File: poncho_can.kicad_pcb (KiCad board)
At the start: 2 copper layers, 85.7 x 60.3 mm, 33 parts, among them J10 GS2, J101 DB9_Male_MountingHoles, J102 DB9_Male_MountingHoles, J103 GS2, J104 GS2, J105 GS2, J106 GS2, J7 GS2, J8 GS2, J9 GS2, U101 TJA1051T, U102 TJA1051T

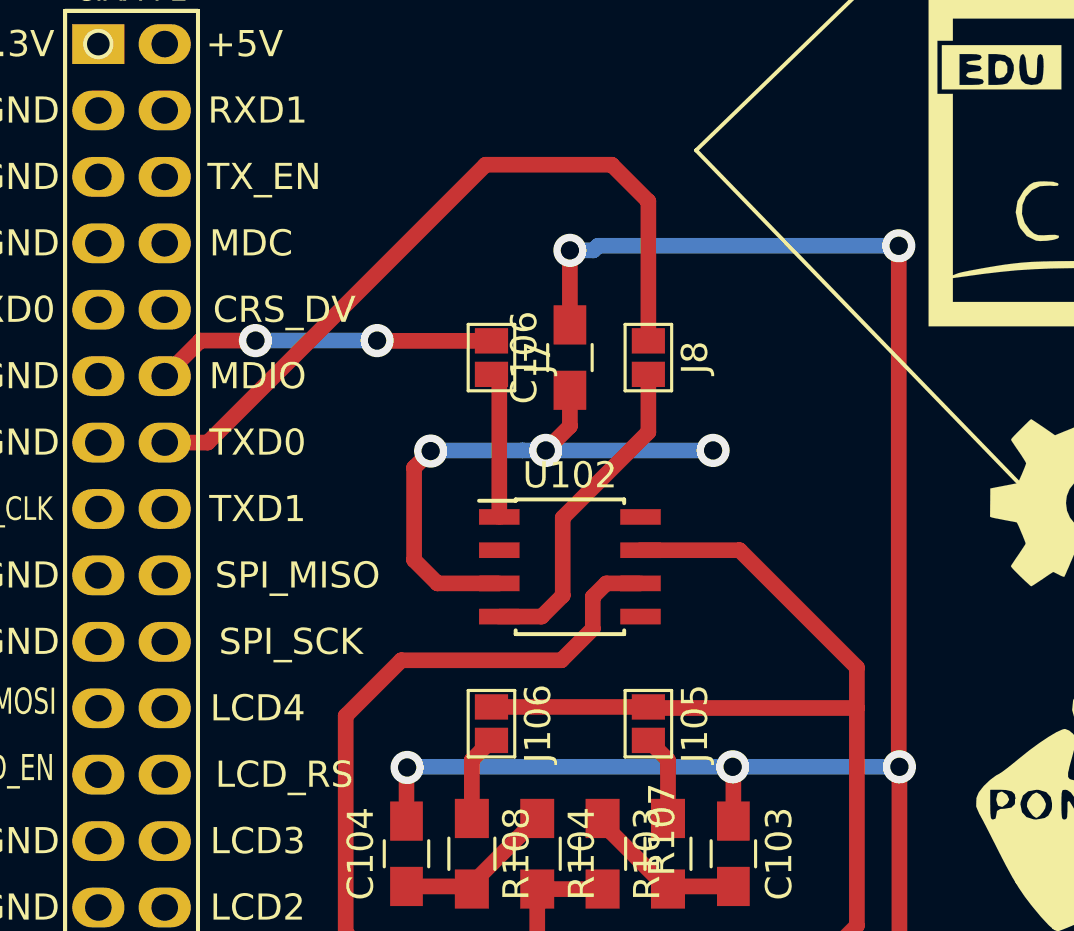
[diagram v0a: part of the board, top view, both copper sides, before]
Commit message: Improved PCB
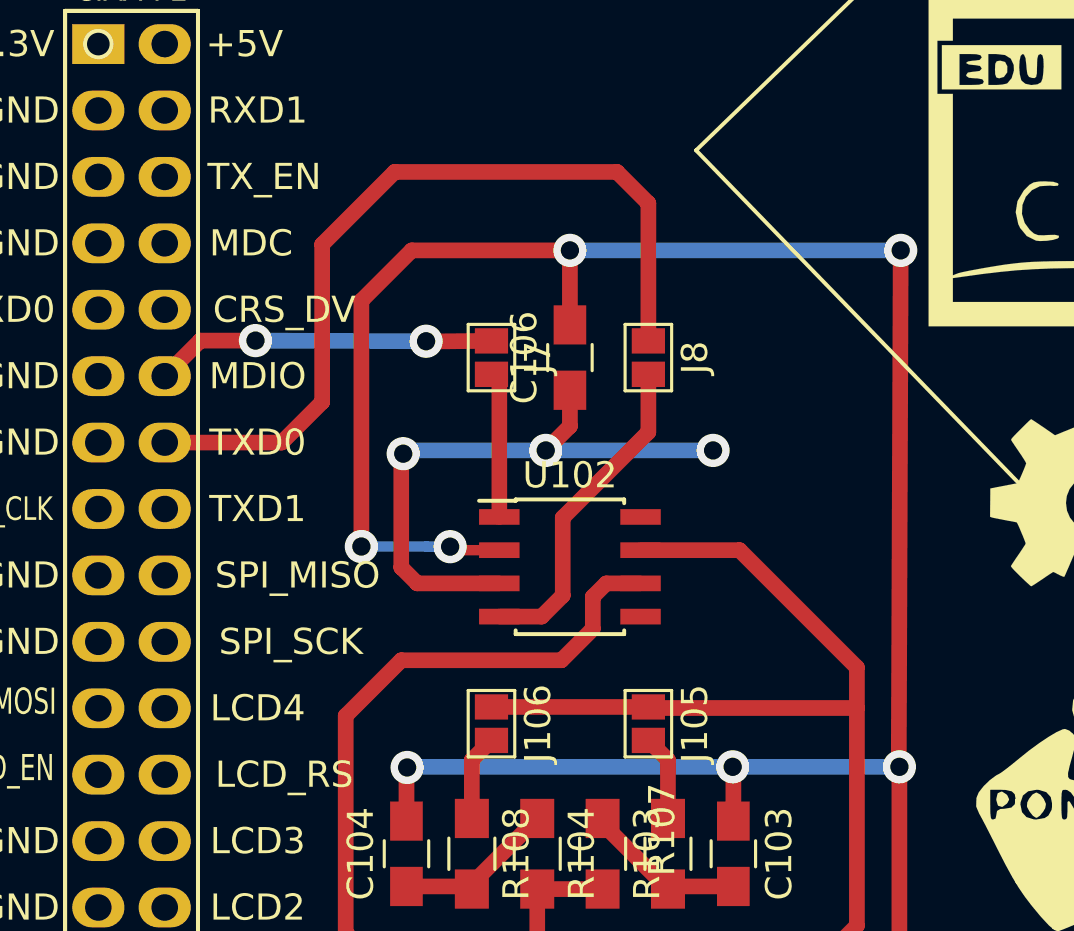
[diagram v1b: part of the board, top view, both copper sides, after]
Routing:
- net GND: track 102.3 -> 125.6 mm, vias 7 -> 9
- net Net-(J8-Pad1): track 28.8 -> 32.1 mm
- net +5V: track 21.6 -> 23.0 mm
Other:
- net class Default: trace_width 0.4 -> 0.6
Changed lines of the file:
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@@
   (general
     (links 77)
-    (no_connects 61)
-    (area 17.572141 15.774999 279.500001 169.160001)
+    (no_connects 53)
+    (area 17.572141 15.774999 279.500001 169.310001)
     (thickness 1.6)
     (drawings 35)
-    (tracks 101)
+    (tracks 111)
     (zones 0)
     (modules 33)
@@
   (net_class Default "This is the default net class."
     (clearance 0.4)
-    (trace_width 0.4)
+    (trace_width 0.6)
     (via_dia 1.27)
     (via_drill 0.7)
@@
     (effects (font (size 1.5 1.5) (thickness 0.3)))
   )
+  (segment (start 83.15 101.9) (end 77.825 101.9) (width 0.6) (layer B.Cu) (net 1))
+  (segment (start 78.235 106.985) (end 81.375 106.985) (width 0.6) (layer F.Cu) (net 1))
+  (segment (start 77.625 106.375) (end 78.235 106.985) (width 0.6) (layer F.Cu) (net 1))
+  (segment (start 77.625 102.075) (end 77.625 106.375) (width 0.6) (layer F.Cu) (net 1))
+  (segment (start 77.7 102) (end 77.625 102.075) (width 0.6) (layer F.Cu) (net 1))
+  (segment (start 77.7 102.025) (end 77.7 102) (width 0.6) (layer F.Cu) (net 1))
+  (via (at 77.7 102.025) (size 1.27) (drill 0.7) (layers F.Cu B.Cu) (net 1))
+  (segment (start 77.825 101.9) (end 77.7 102.025) (width 0.6) (layer B.Cu) (net 1))
   (segment (start 83.15 101.9) (end 89.55 101.9) (width 0.6) (layer B.Cu) (net 1))
   (via (at 89.55 101.9) (size 1.27) (drill 0.7) (layers F.Cu B.Cu) (net 1))
-  (segment (start 78.115001 106.090001) (end 79.01 106.985) (width 0.6) (layer F.Cu) (net 1))
-  (segment (start 79.01 106.985) (end 81.375 106.985) (width 0.6) (layer F.Cu) (net 1))
-  (segment (start 78.75 101.925) (end 78.115001 102.559999) (width 0.6) (layer F.Cu) (net 1))
-  (segment (start 78.115001 102.559999) (end 78.115001 106.090001) (width 0.6) (layer F.Cu) (net 1))
-  (segment (start 82.251975 101.9) (end 78.775 101.9) (width 0.6) (layer B.Cu) (net 1))
-  (segment (start 78.775 101.9) (end 78.75 101.925) (width 0.6) (layer B.Cu) (net 1))
-  (via (at 78.75 101.925) (size 1.27) (drill 0.7) (layers F.Cu B.Cu) (net 1))
-  (segment (start 83.15 101.9) (end 82.251975 101.9) (width 0.6) (layer B.Cu) (net 1))
   (segment (start 84.075 99.6) (end 84.075 100.975) (width 0.6) (layer F.Cu) (net 1))
   (segment (start 84.075 100.975) (end 83.15 101.9) (width 0.6) (layer F.Cu) (net 1))
   (via (at 83.15 101.9) (size 1.27) (drill 0.7) (layers F.Cu B.Cu) (net 1))
-  (segment (start 96.65 94.075) (end 96.65 113.975) (width 0.6) (layer F.Cu) (net 2))
+  (segment (start 84.075 94.25) (end 96.725 94.25) (width 0.6) (layer B.Cu) (net 2))
+  (segment (start 96.725 94.25) (end 96.65 113.975) (width 0.6) (layer F.Cu) (net 2))
+  (via (at 84.075 94.25) (size 1.27) (drill 0.7) (layers F.Cu B.Cu) (net 2))
+  (via (at 96.725 94.25) (size 1.27) (drill 0.7) (layers F.Cu B.Cu) (net 2))
   (segment (start 96.65 113.975) (end 96.675 114) (width 0.6) (layer F.Cu) (net 2))
-  (segment (start 85.148025 94.075) (end 96.65 94.075) (width 0.6) (layer B.Cu) (net 2))
-  (via (at 96.65 94.075) (size 1.27) (drill 0.7) (layers F.Cu B.Cu) (net 2))
-  (segment (start 84.075 94.25) (end 84.973025 94.25) (width 0.6) (layer B.Cu) (net 2))
-  (segment (start 84.973025 94.25) (end 85.148025 94.075) (width 0.6) (layer B.Cu) (net 2))
+  (segment (start 76.1 105.575) (end 76.1 96.175) (width 0.6) (layer F.Cu) (net 2))
+  (segment (start 79.627976 105.715) (end 79.493988 105.581012) (width 0.4) (layer F.Cu) (net 2))
+  (via (at 79.493988 105.581012) (size 1.27) (drill 0.7) (layers F.Cu B.Cu) (net 2))
+  (segment (start 81.375 105.715) (end 79.627976 105.715) (width 0.4) (layer F.Cu) (net 2))
+  (segment (start 78.595963 105.581012) (end 78.589951 105.575) (width 0.4) (layer B.Cu) (net 2))
+  (segment (start 79.493988 105.581012) (end 78.595963 105.581012) (width 0.4) (layer B.Cu) (net 2))
+  (via (at 76.1 105.575) (size 1.27) (drill 0.7) (layers F.Cu B.Cu) (net 2))
+  (segment (start 78.589951 105.575) (end 76.1 105.575) (width 0.4) (layer B.Cu) (net 2))
+  (segment (start 78.025 94.25) (end 84.075 94.25) (width 0.6) (layer F.Cu) (net 2))
+  (segment (start 76.1 96.175) (end 78.025 94.25) (width 0.6) (layer F.Cu) (net 2))
   (segment (start 84.075 97.1) (end 84.075 94.25) (width 0.6) (layer F.Cu) (net 2))
-  (via (at 84.075 94.25) (size 1.27) (drill 0.7) (layers F.Cu B.Cu) (net 2))
   (segment (start 96.675 114) (end 96.675 125.05) (width 0.6) (layer F.Cu) (net 2))
   (segment (start 96.675 125.05) (end 96.6 125.125) (width 0.6) (layer F.Cu) (net 2))
@@
   (segment (start 69.94 97.7) (end 68.58 99.06) (width 0.6) (layer F.Cu) (net 57))
   (via (at 72.05 97.7) (size 1.27) (drill 0.7) (layers F.Cu B.Cu) (net 57))
-  (segment (start 76.7 97.7) (end 72.05 97.7) (width 0.6) (layer B.Cu) (net 57))
-  (segment (start 81.075 97.71) (end 76.71 97.71) (width 0.6) (layer F.Cu) (net 57))
-  (segment (start 76.71 97.71) (end 76.7 97.7) (width 0.6) (layer F.Cu) (net 57))
-  (via (at 76.7 97.7) (size 1.27) (drill 0.7) (layers F.Cu B.Cu) (net 57))
+  (segment (start 78.575 97.725) (end 72.05 97.7) (width 0.6) (layer B.Cu) (net 57))
+  (segment (start 81.075 97.71) (end 78.585 97.735) (width 0.6) (layer F.Cu) (net 57))
+  (segment (start 78.585 97.735) (end 78.575 97.725) (width 0.6) (layer F.Cu) (net 57))
+  (via (at 78.575 97.725) (size 1.27) (drill 0.7) (layers F.Cu B.Cu) (net 57))
   (segment (start 81.375 104.445) (end 81.375 99.29) (width 0.6) (layer F.Cu) (net 58))
   (segment (start 81.375 99.29) (end 81.075 98.99) (width 0.6) (layer F.Cu) (net 58))
-  (segment (start 80.85 90.975) (end 70.225 101.6) (width 0.6) (layer F.Cu) (net 59))
-  (segment (start 70.225 101.6) (end 68.58 101.6) (width 0.6) (layer F.Cu) (net 59))
-  (segment (start 85.675 90.975) (end 80.85 90.975) (width 0.6) (layer F.Cu) (net 59))
-  (segment (start 87.075 92.375) (end 85.675 90.975) (width 0.6) (layer F.Cu) (net 59))
-  (segment (start 87.075 97.71) (end 87.075 92.375) (width 0.6) (layer F.Cu) (net 59))
+  (segment (start 87.075 97.71) (end 87.075 92.45) (width 0.6) (layer F.Cu) (net 59))
+  (segment (start 73.05 101.6) (end 68.58 101.6) (width 0.6) (layer F.Cu) (net 59))
+  (segment (start 74.6 100.05) (end 73.05 101.6) (width 0.6) (layer F.Cu) (net 59))
+  (segment (start 74.6 94.025) (end 74.6 100.05) (width 0.6) (layer F.Cu) (net 59))
+  (segment (start 77.375 91.25) (end 74.6 94.025) (width 0.6) (layer F.Cu) (net 59))
+  (segment (start 85.875 91.25) (end 77.375 91.25) (width 0.6) (layer F.Cu) (net 59))
+  (segment (start 87.075 92.45) (end 85.875 91.25) (width 0.6) (layer F.Cu) (net 59))
   (segment (start 87.075 98.99) (end 87.075 101.2) (width 0.6) (layer F.Cu) (net 60))
   (segment (start 82.995 108.255) (end 81.375 108.255) (width 0.6) (layer F.Cu) (net 60))
